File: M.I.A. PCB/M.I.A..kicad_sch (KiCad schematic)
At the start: 41 parts, among them J1 USB_C_Receptacle_USB2.0_16P, SW1 SW_Push, SW2 SW_Push, U1 W25Q128JVS, U2 RP2350B-QFN80, Y1 ABM8-272-T3

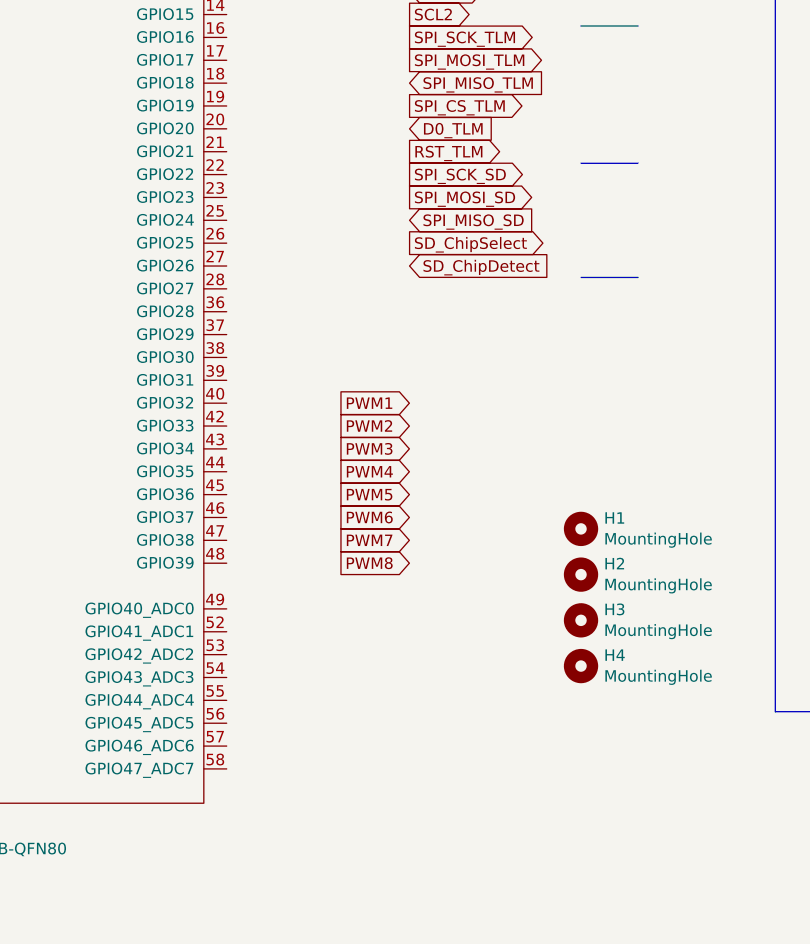
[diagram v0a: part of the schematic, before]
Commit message: Worked More on Layout/Wiring
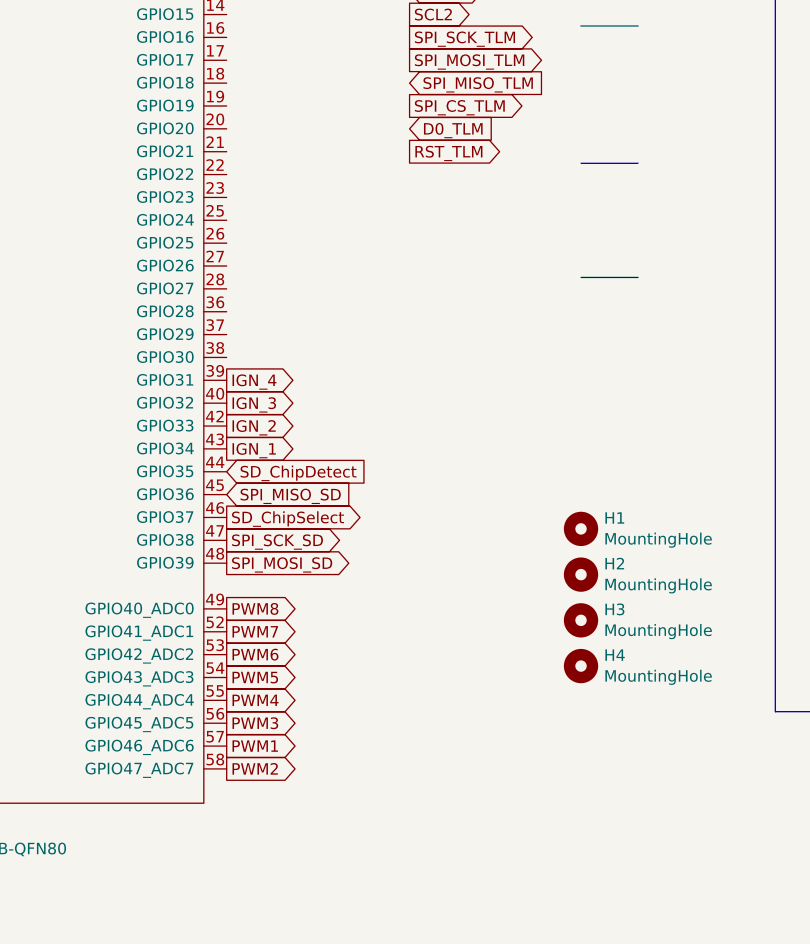
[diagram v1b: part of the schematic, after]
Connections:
- net PWM1: now also U2.57 (GPIO46_ADC6)
- net PWM2: now also U2.58 (GPIO47_ADC7)
- net PWM3: now also U2.56 (GPIO45_ADC5)
- net PWM4: now also U2.55 (GPIO44_ADC4)
- net PWM5: now also U2.54 (GPIO43_ADC3)
- net PWM6: now also U2.53 (GPIO42_ADC2)
- net PWM7: now also U2.52 (GPIO41_ADC1)
- net PWM8: now also U2.49 (GPIO40_ADC0)
- net SD_ChipDetect: now also U2.44 (GPIO35)
- net SD_ChipSelect: now also U2.46 (GPIO37)
- net SPI_MISO_SD: now also U2.45 (GPIO36)
- net SPI_MOSI_SD: now also U2.48 (GPIO39)
- net SPI_SCK_SD: now also U2.47 (GPIO38)
- net IGN_4: now reaches U2.39 (GPIO31)
- net IGN_3: now reaches U2.40 (GPIO32)
- net IGN_2: now reaches U2.42 (GPIO33)
- net IGN_1: now reaches U2.43 (GPIO34)
